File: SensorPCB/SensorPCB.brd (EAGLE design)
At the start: 37 x 65 mm, 31 parts, among them T1 33u

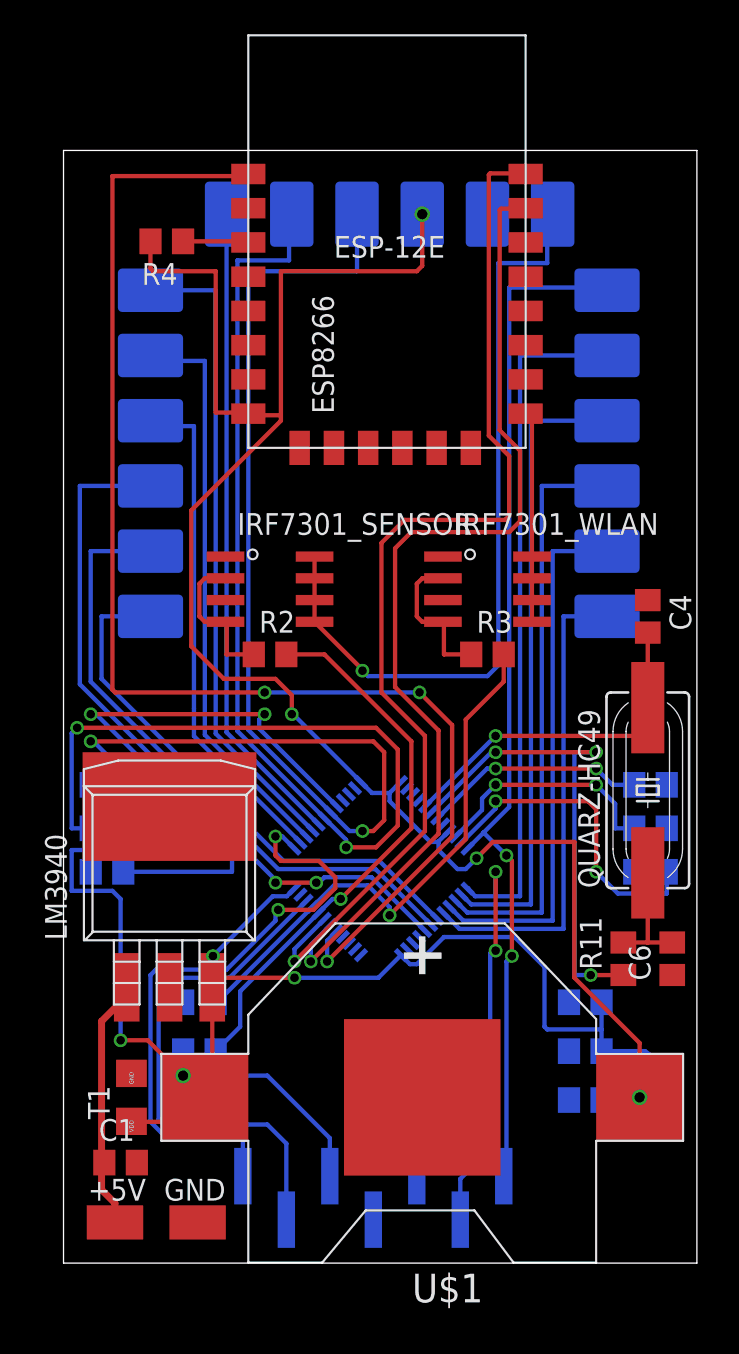
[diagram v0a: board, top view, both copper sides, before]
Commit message: some changes
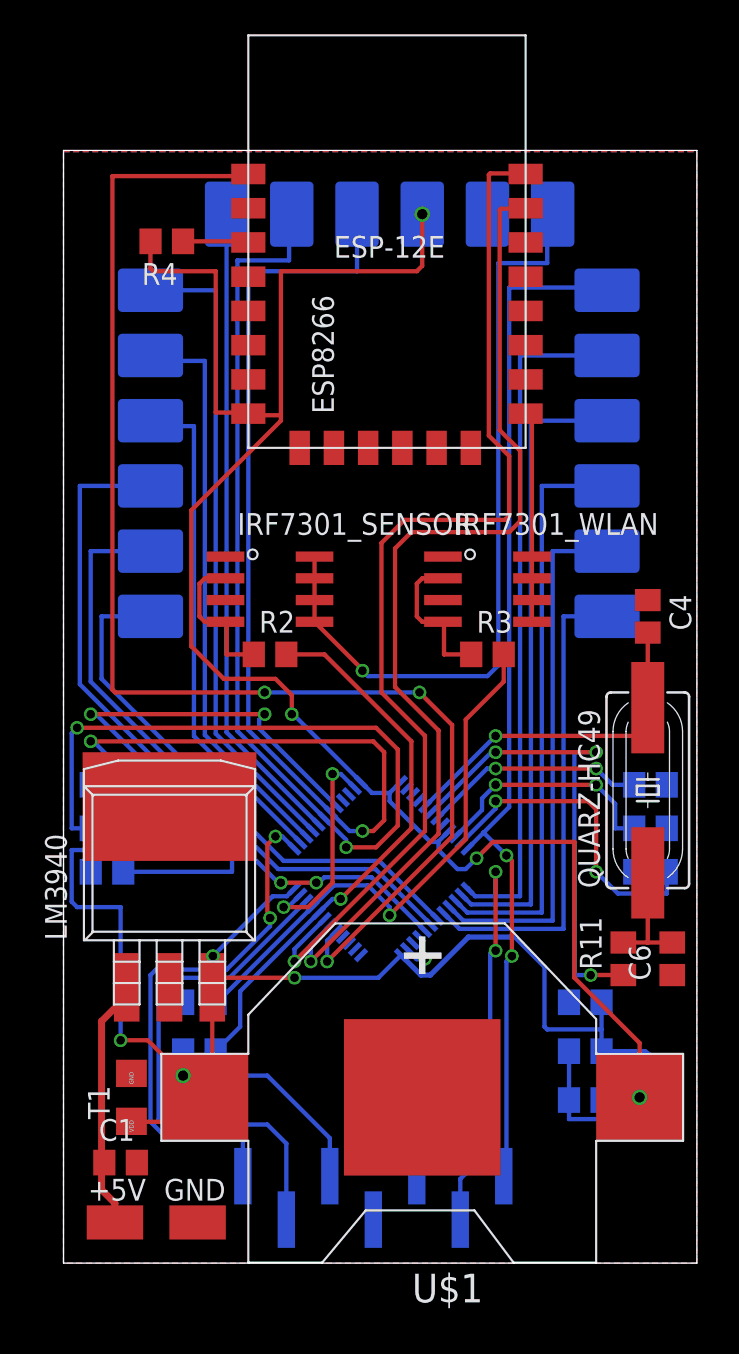
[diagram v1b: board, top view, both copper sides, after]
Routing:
- net GND: track 0.00 -> 25.0 mm, vias 0 -> 3
- net SWCLK: track 37.0 -> 31.8 mm
- net +3V3: track 208.5 -> 209.0 mm
- added copper zone on layer 1, net GND
- added copper zone on layer 16, net GND
